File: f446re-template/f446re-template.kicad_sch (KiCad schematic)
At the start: 36 parts, among them J1 電源コネクタ, J2 デバッグ端子, J3 CANコネクタ, SW1 リセットスイッチ, U1 AZ1117-3.3, U2 STM32F446RETx, U3 MCP2562-E-SN, Y1 16MHz

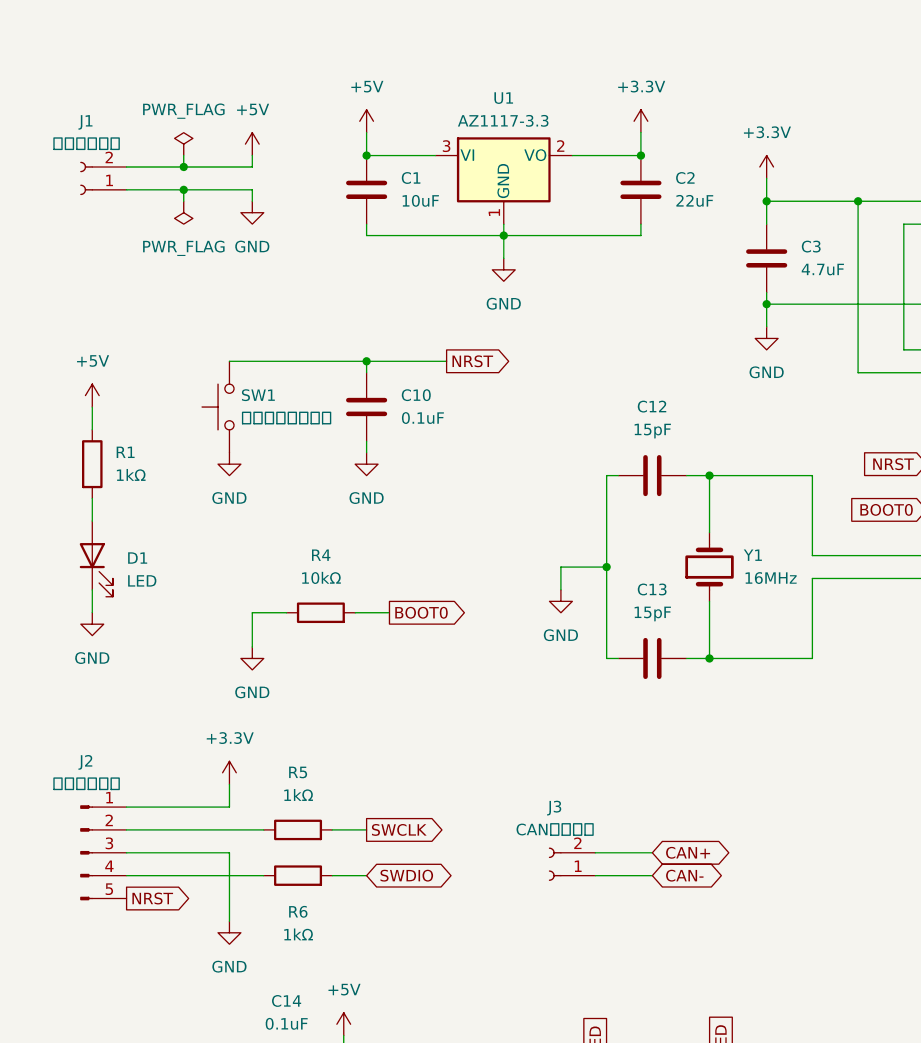
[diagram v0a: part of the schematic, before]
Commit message: 2025/06/09/23:25
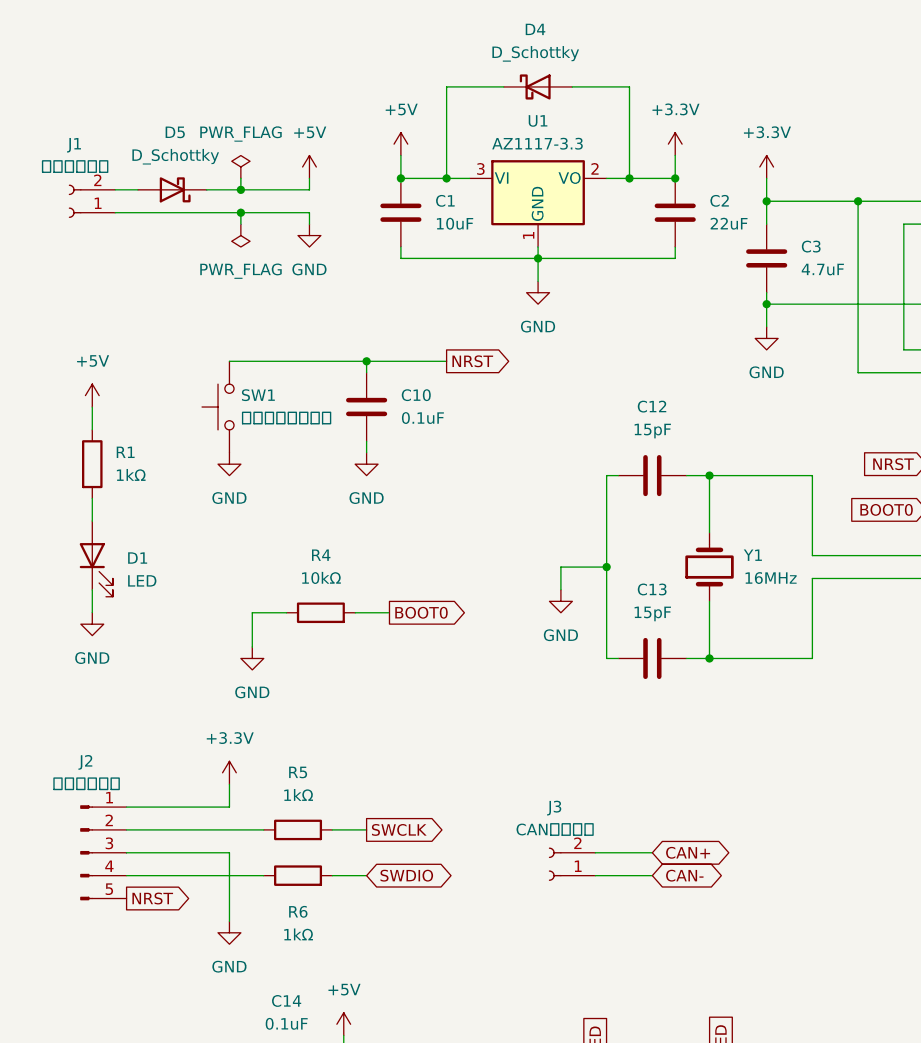
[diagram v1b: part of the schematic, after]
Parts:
- added D4, D5: D_Schottky, my_library:US2H, symbol Device:D_Schottky
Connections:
- net +3.3V: now also D4.2 (A)
- net +5V: now also D4.1 (K), D5.1 (K); no longer J1.2 (Pin_2)
- new net: D5.2 (A), J1.2 (Pin_2)
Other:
- moved on the sheet: C1, C2, J1, U1
